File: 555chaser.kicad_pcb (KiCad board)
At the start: 2 copper layers, 99.6 x 90.3 mm, 18 parts, among them J1 Conn_01x02_Socket, U1 NE555P, U2 4017

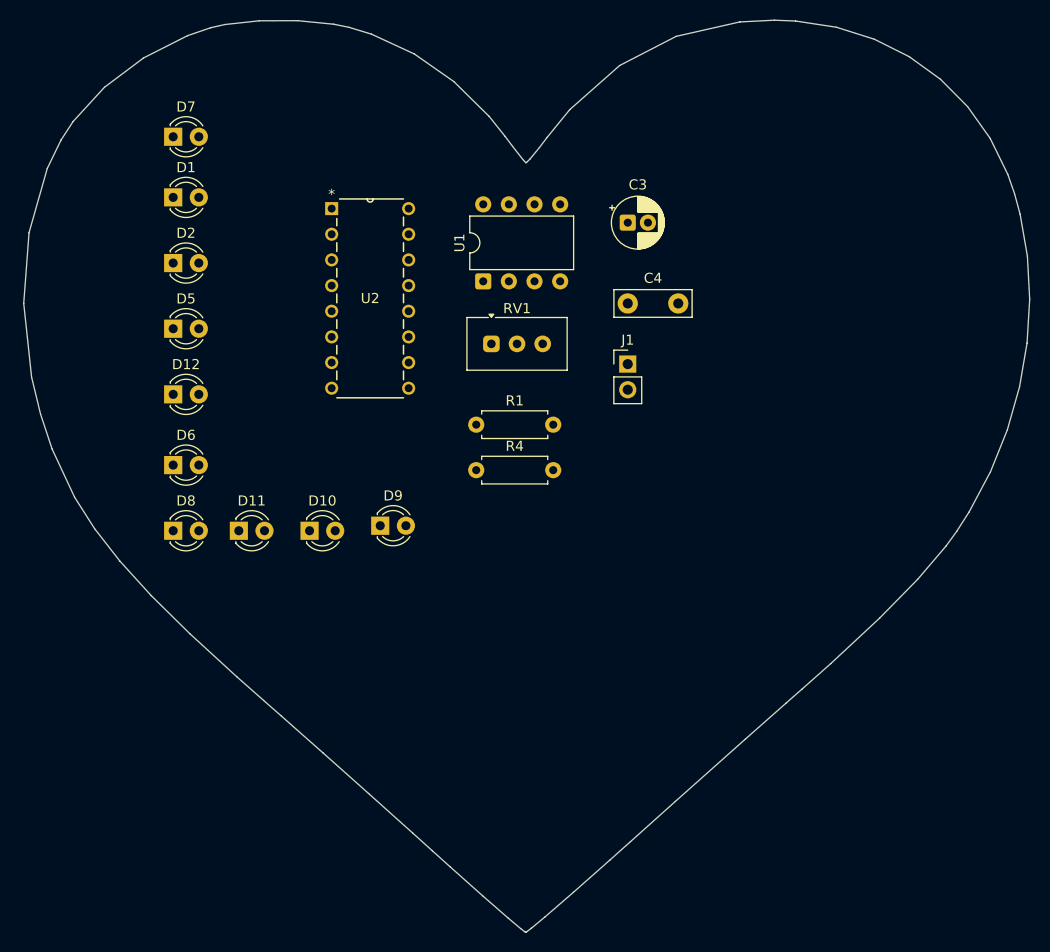
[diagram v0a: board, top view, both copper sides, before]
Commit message: Add files via upload
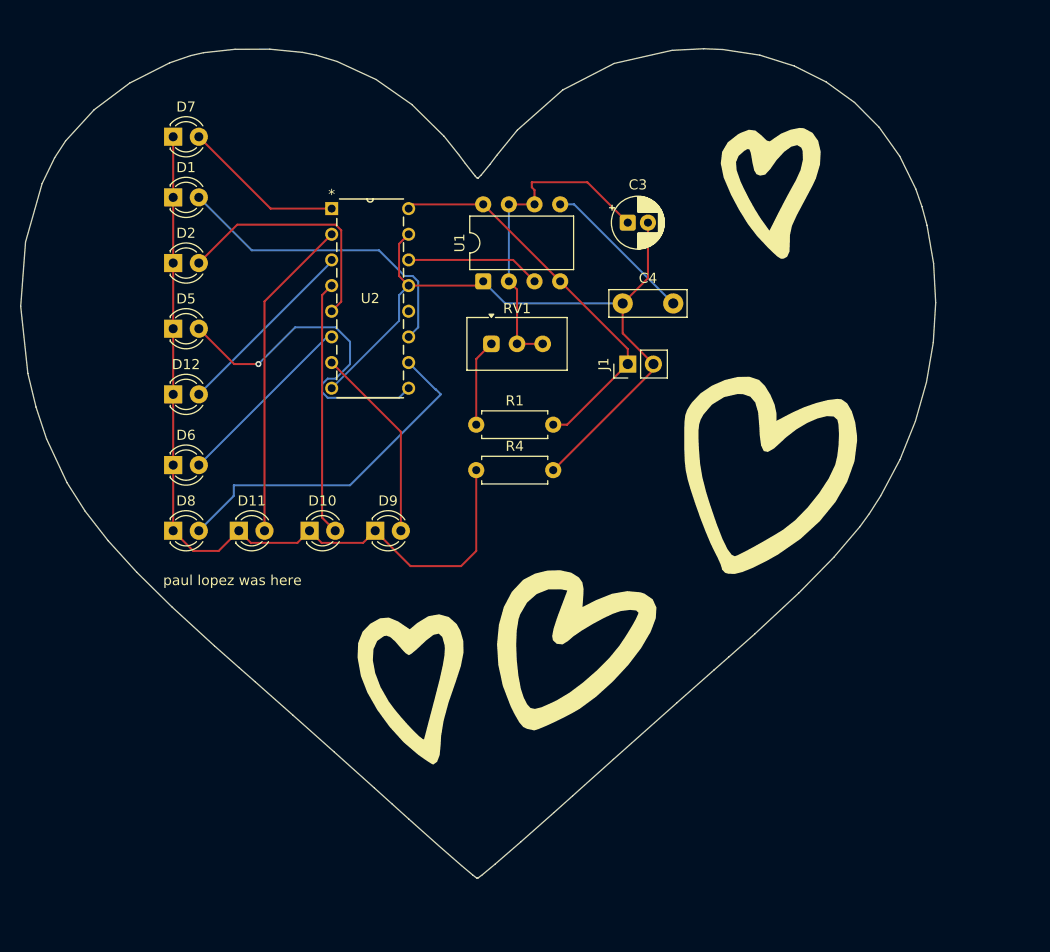
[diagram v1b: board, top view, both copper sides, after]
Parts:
- added G***: LOGO, footprints:layla, F.Cu at (154.5, 108.0)
- moved D9 0.71 mm to (140.5, 118.0)
- moved C4 0.50 mm to (165.0, 95.5)
- turned J1 to 90 degrees
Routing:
- net Net-(D1-K): track 0.00 -> 82.7 mm
- net GND: track 0.00 -> 72.4 mm
- net +5V: track 0.00 -> 39.2 mm
- net Net-(D8-A): track 0.00 -> 34.7 mm
- net Net-(D5-A): track 0.00 -> 34.3 mm, vias 0 -> 1
- net TR: track 0.00 -> 32.7 mm
- net Net-(D11-A): track 0.00 -> 32.1 mm
- net Net-(D1-A): track 0.00 -> 31.0 mm
- net Net-(D10-A): track 0.00 -> 25.2 mm
- net Net-(D2-A): track 0.00 -> 24.3 mm
- net Net-(D9-A): track 0.00 -> 19.5 mm
- net Net-(D12-A): track 0.00 -> 18.8 mm
- net Net-(D6-A): track 0.00 -> 18.4 mm
- net Net-(D7-A): track 0.00 -> 16.1 mm
- net Net-(U1-CONT): track 0.00 -> 15.3 mm
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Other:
- board size 99.6 x 90.3 mm -> 90.6 x 82.1 mm
- board text added: "paul lopez was here"
